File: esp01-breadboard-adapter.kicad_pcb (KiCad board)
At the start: 2 copper layers, 4 parts, among them P1 CONN_02X04, P2 CONN_01X04, P3 CONN_01X04

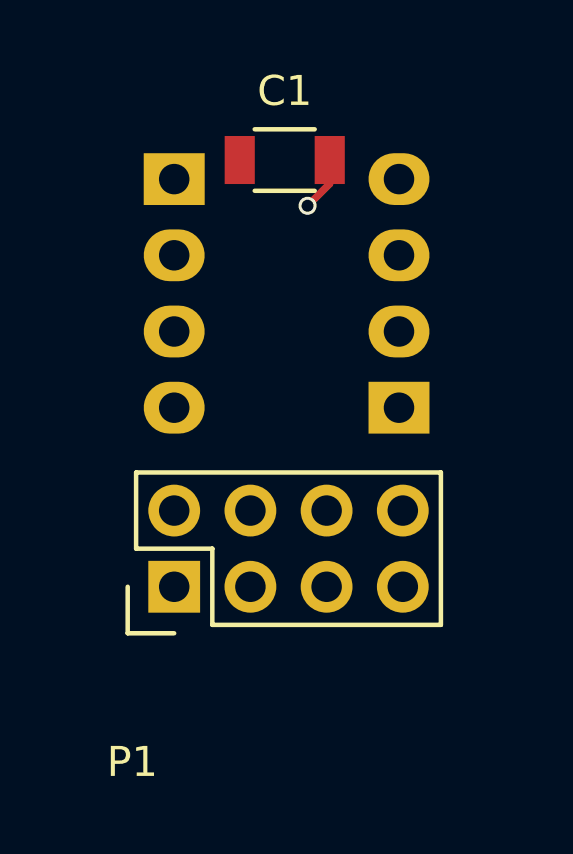
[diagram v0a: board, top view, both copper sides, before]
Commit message: pcb finished
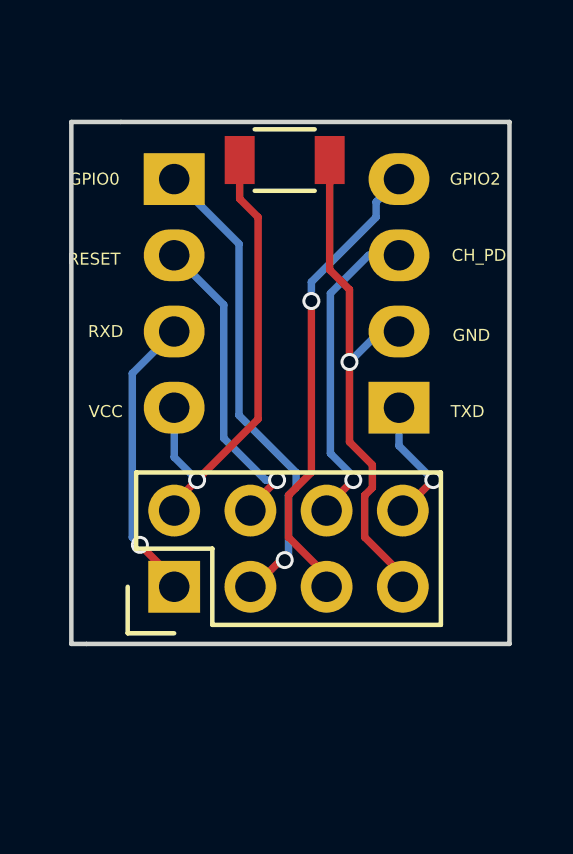
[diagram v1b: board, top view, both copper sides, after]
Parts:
- C1: value C -> 100u
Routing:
- net GND: track 1.96 -> 18.4 mm
- net GPIO0: track 0.38 -> 16.4 mm, vias 0 -> 1
- net VCC: track 0.00 -> 15.8 mm, vias 0 -> 1
- net GPIO2: track 0.38 -> 16.1 mm, vias 0 -> 1
- net CH_PD: track 0.00 -> 10.7 mm, vias 0 -> 1
- net RESET: track 0.32 -> 10.8 mm, vias 0 -> 1
- net RXD: track 1.27 -> 10.9 mm, vias 0 -> 1
- net TXD: track 0.18 -> 4.50 mm, vias 0 -> 1
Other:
- board outline added: 14.6 x 17.4 mm
- board text added: "CH_PD"
- board text added: "GND"
- board text added: "GPIO0"
- board text added: "GPIO2"
- board text added: "RESET"
- board text added: "RXD"
- board text added: "TXD"
- board text added: "VCC"
